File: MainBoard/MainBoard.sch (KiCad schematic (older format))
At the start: 6 parts

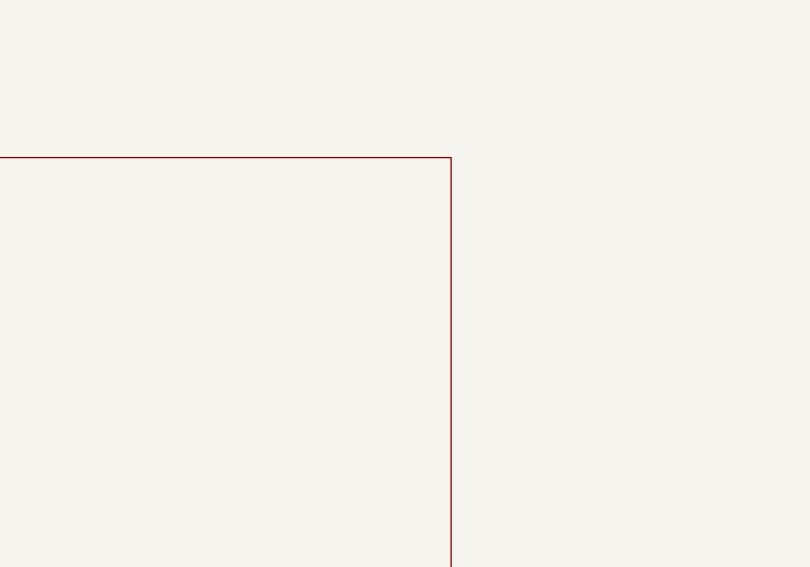
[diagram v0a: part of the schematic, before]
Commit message: add hierachy pins
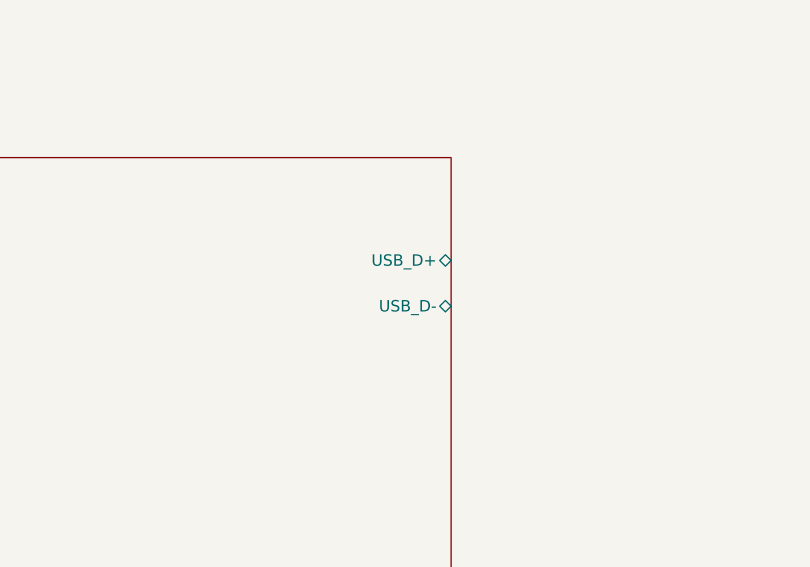
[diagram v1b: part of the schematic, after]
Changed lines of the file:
@@
 F0 "keyboard" 50
 F1 "keyboard.sch" 50
+F2 "USB_D+" B R 10700 12500 50
+F3 "USB_D-" B R 10700 12700 50
 $EndSheet
 $EndSCHEMATC

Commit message: add hierachy pins
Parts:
- removed J?: Conn_Coaxial, symbol Connector:Conn_Coaxial
- J?: value DF40C-100DS-0.4V(51) -> DF40C-100DS-0.4V(51) _LFT
- J?: value DF40C-100DS-0.4V(51) -> DF40C-100DS-0.4V(51) _RFT
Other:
- moved on the sheet: J?
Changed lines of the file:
@@
-$EndComp
-$Comp
-L Connector:Conn_Coaxial J?
-U 1 1 60395F77
-P 21200 7000
-F 0 "J?" H 21300 6975 50  0000 L CNN
-F 1 "Conn_Coaxial" H 21300 6884 50  0000 L CNN
-F 2 "" H 21200 7000 50  0001 C CNN
-F 3 " ~" H 21200 7000 50  0001 C CNN
-	1    21200 7000
-	1    0    0    -1
 $EndComp
 $Comp
@@
 P 4850 3750
 F 0 "J?" H 4850 6417 50  0000 C CNN
-F 1 "DF40C-100DS-0.4V(51)" H 4850 6326 50  0000 C CNN
+F 1 "DF40C-100DS-0.4V(51) _LFT" H 4850 6326 50  0000 C CNN
 F 2 "HRS_DF40C-100DS-0.4V(51)" H 4850 3750 50  0001 L BNN
 F 3 "" H 4850 3750 50  0001 L BNN
@@
 L DF40C-100DS-0.4V_51_:DF40C-100DS-0.4V(51) J?
 U 1 1 6039B9F7
-P 9300 3750
-F 0 "J?" H 9300 6417 50  0000 C CNN
-F 1 "DF40C-100DS-0.4V(51)" H 9300 6326 50  0000 C CNN
-F 2 "HRS_DF40C-100DS-0.4V(51)" H 9300 3750 50  0001 L BNN
-F 3 "" H 9300 3750 50  0001 L BNN
-F 4 "HRS" H 9300 3750 50  0001 L BNN "MF"
-F 5 "None" H 9300 3750 50  0001 L BNN "PACKAGE"
-F 6 "Good" H 9300 3750 50  0001 L BNN "AVAILABILITY"
-F 7 "$1.36 USD" H 9300 3750 50  0001 L BNN "PRICE"
-F 8 "DF40C-100DS-0.4V(51)" H 9300 3750 50  0001 L BNN "MP"
-	1    9300 3750
+P 8450 3750
+F 0 "J?" H 8450 6417 50  0000 C CNN
+F 1 "DF40C-100DS-0.4V(51) _RFT" H 8450 6326 50  0000 C CNN
+F 2 "HRS_DF40C-100DS-0.4V(51)" H 8450 3750 50  0001 L BNN
+F 3 "" H 8450 3750 50  0001 L BNN
+F 4 "HRS" H 8450 3750 50  0001 L BNN "MF"
+F 5 "None" H 8450 3750 50  0001 L BNN "PACKAGE"
+F 6 "Good" H 8450 3750 50  0001 L BNN "AVAILABILITY"
+F 7 "$1.36 USD" H 8450 3750 50  0001 L BNN "PRICE"
+F 8 "DF40C-100DS-0.4V(51)" H 8450 3750 50  0001 L BNN "MP"
+	1    8450 3750
 	1    0    0    -1
 $EndComp
